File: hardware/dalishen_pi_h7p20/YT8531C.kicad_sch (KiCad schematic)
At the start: 48 parts, among them J10 RJ45_HR911130A, U1 YT8531C, Y2 NC

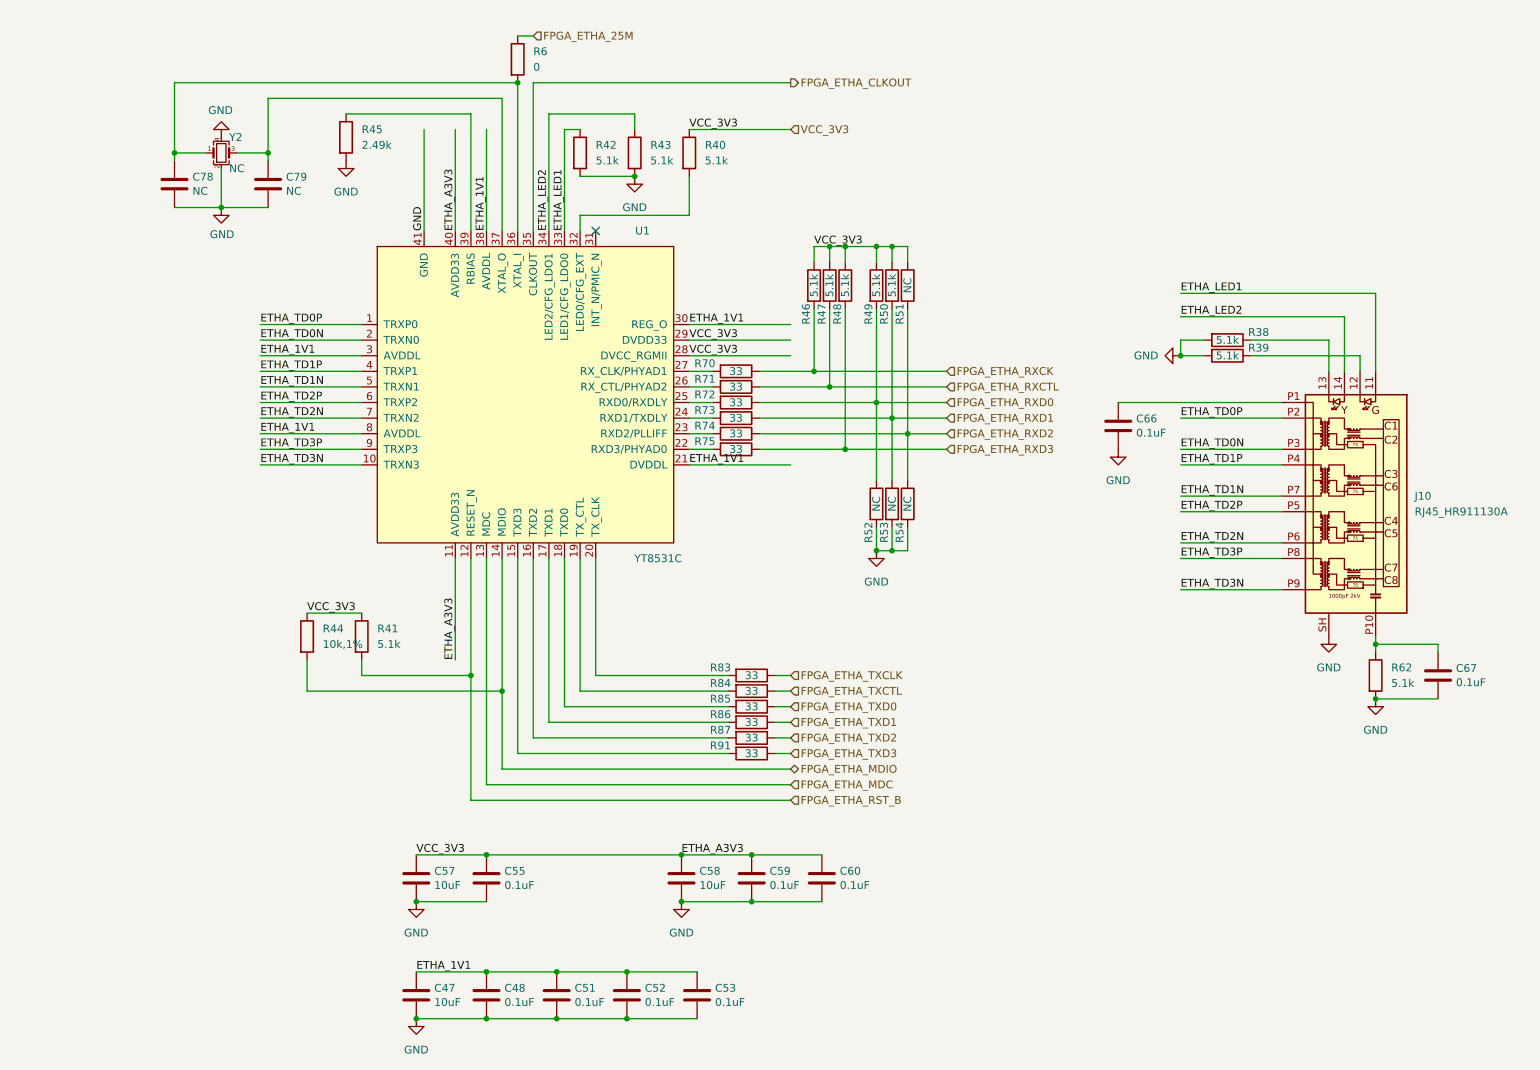
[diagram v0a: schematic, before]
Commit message: [dalishen_pi_h7p20] layout done
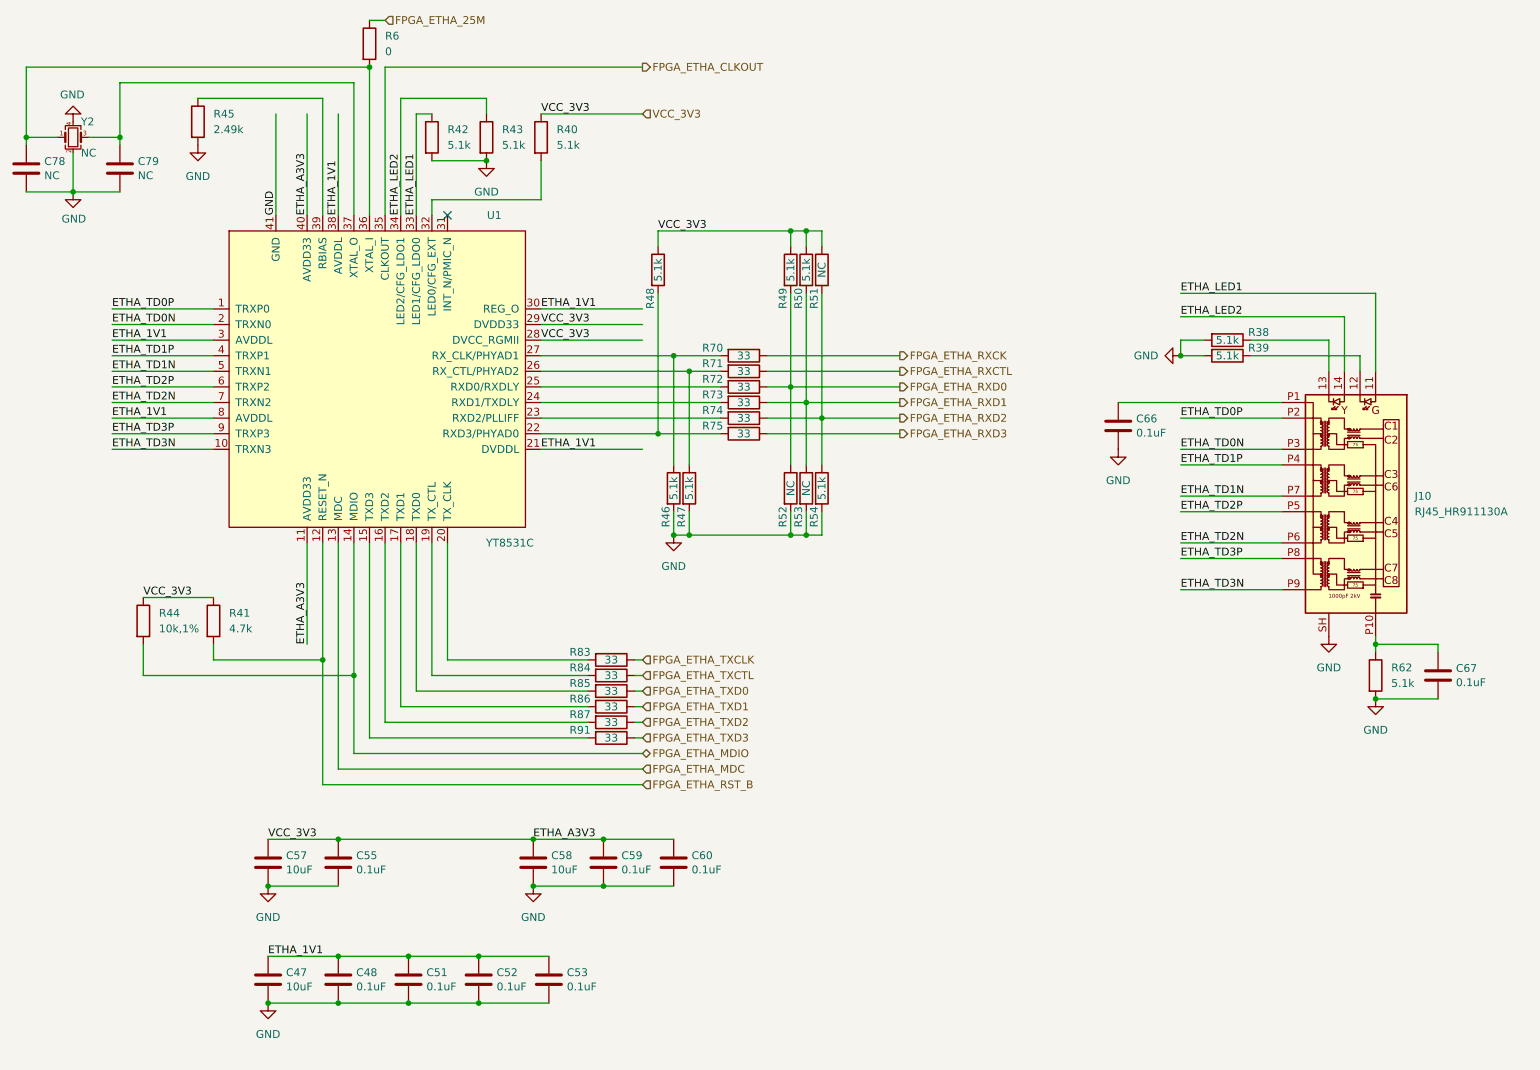
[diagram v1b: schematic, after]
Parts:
- R41: value 5.1k -> 4.7k
- R54: value NC -> 5.1k
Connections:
- net FPGA_ETHA_RXCK: no longer R46.2
- net FPGA_ETHA_RXCTL: no longer R47.2
- net FPGA_ETHA_RXD3: no longer R48.2
- net GND: now also R46.2, R47.2
- net VCC_3V3: no longer R46.1, R47.1
- net at R75.2, U1.22 (RXD3/PHYAD0): now also R48.2
- net at R71.2, U1.26 (RX_CTL/PHYAD2): now also R47.1
- net at R70.2, U1.27 (RX_CLK/PHYAD1): now also R46.1
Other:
- moved on the sheet: C47, C48, C51, C52, C53, C55, C57, C58, C59, C60, C78, C79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
